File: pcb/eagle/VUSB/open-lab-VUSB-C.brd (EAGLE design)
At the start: 69.5 x 58.4 mm, 70 parts, among them IC1 ATMEGA328P, IC2 MCP73831, IC4 MCP1700-33, IC5 MCP23008, IC6 MAX31855, IC7 ENC28J60, J1 AYZ0202, Q1 BSS123, Q2 BSS123, Q3 BSS123, X1 USBSMD, X2 32.768kHz, X3 25MHz

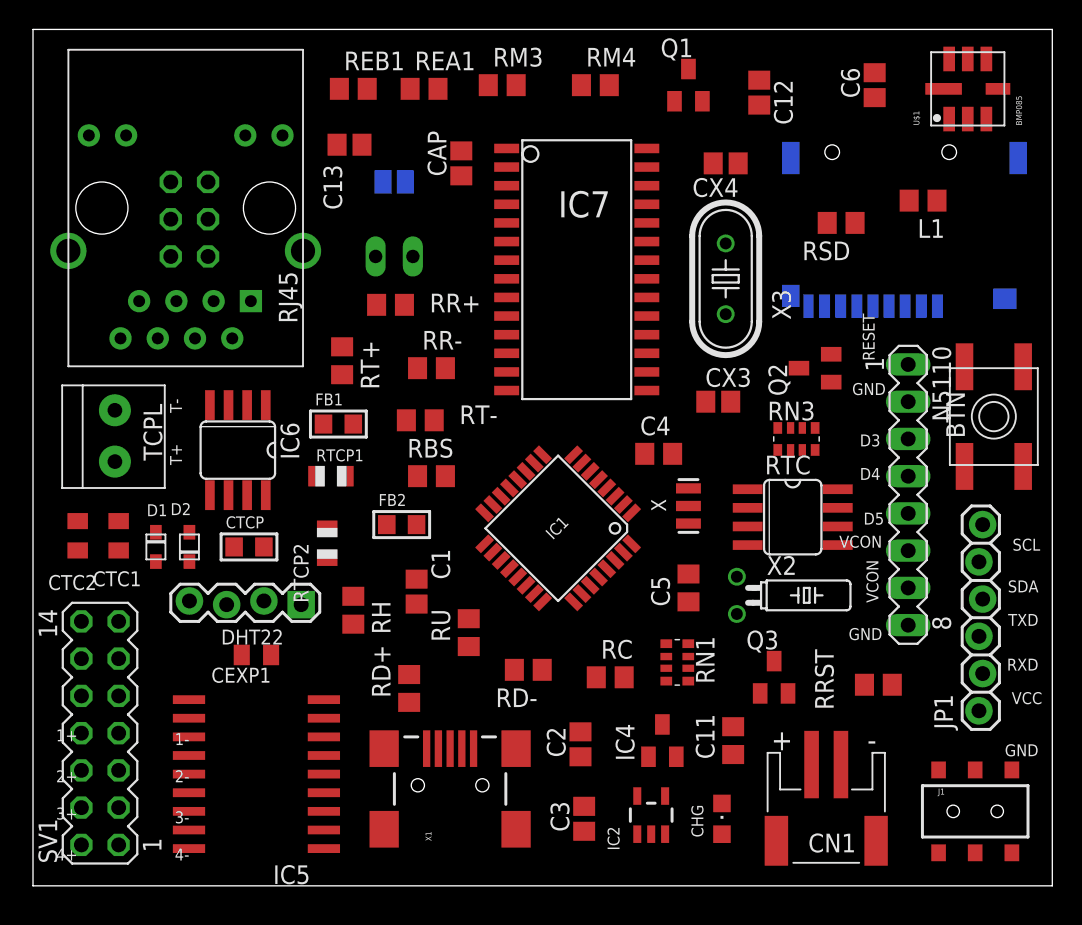
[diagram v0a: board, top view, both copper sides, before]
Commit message: update
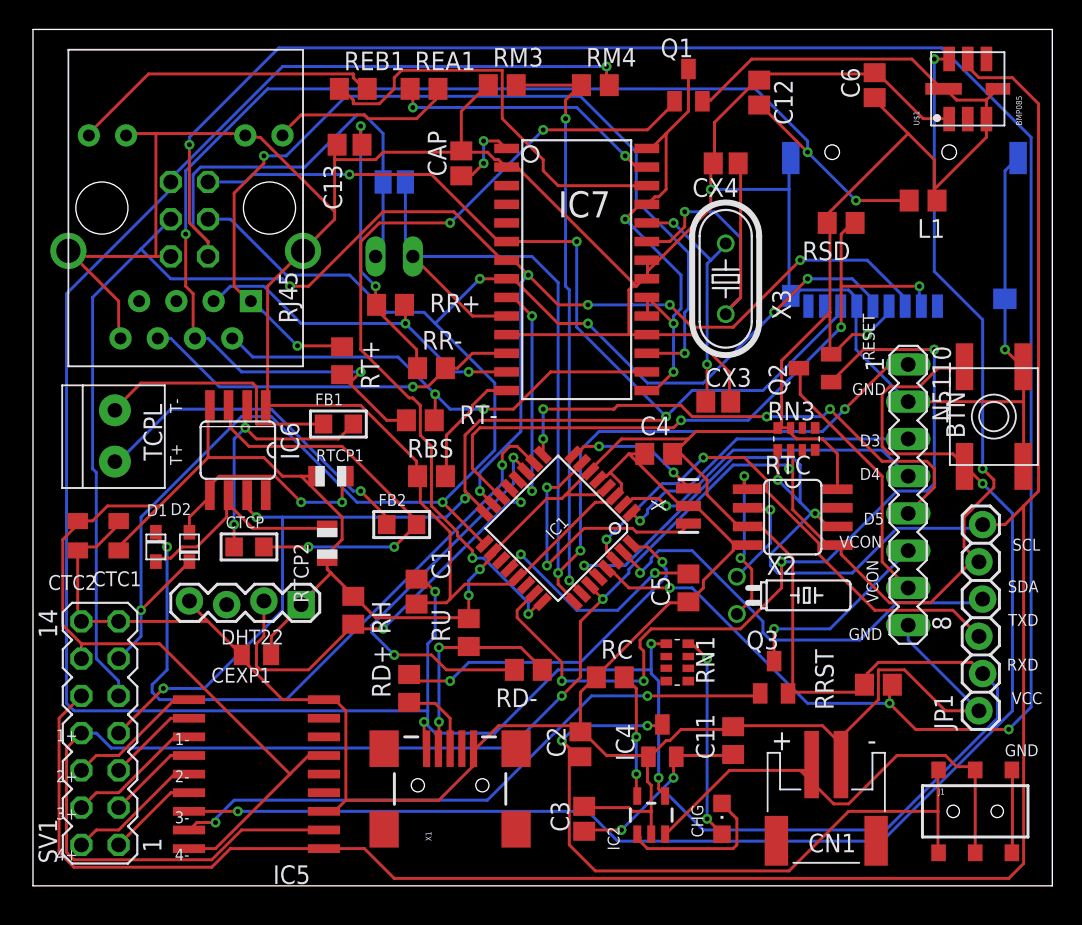
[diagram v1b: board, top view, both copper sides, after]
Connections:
- net GND: now also IC5.4, IC5.5
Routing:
- net GND: track 0.00 -> 391.6 mm, vias 0 -> 2
- net VCC: track 0.00 -> 285.5 mm, vias 0 -> 5
- net SCL: track 0.00 -> 191.3 mm, vias 0 -> 3
- net RESET: track 0.00 -> 175.3 mm, vias 0 -> 4
- net SDA: track 0.00 -> 147.0 mm, vias 0 -> 5
- net VBUS: track 0.00 -> 140.2 mm, vias 0 -> 5
- net SCK: track 0.00 -> 116.7 mm, vias 0 -> 6
- net MISO: track 0.00 -> 114.9 mm, vias 0 -> 6
- net MOSI: track 0.00 -> 114.9 mm, vias 0 -> 6
- net P6: track 0.00 -> 94.9 mm, vias 0 -> 2
- net TCT: track 0.00 -> 91.6 mm, vias 0 -> 4
- net A2: track 0.00 -> 80.0 mm, vias 0 -> 3
- net TD+: track 0.00 -> 65.4 mm, vias 0 -> 3
- net A0: track 0.00 -> 58.8 mm, vias 0 -> 4
- net A1: track 0.00 -> 57.4 mm, vias 0 -> 4
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
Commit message: update
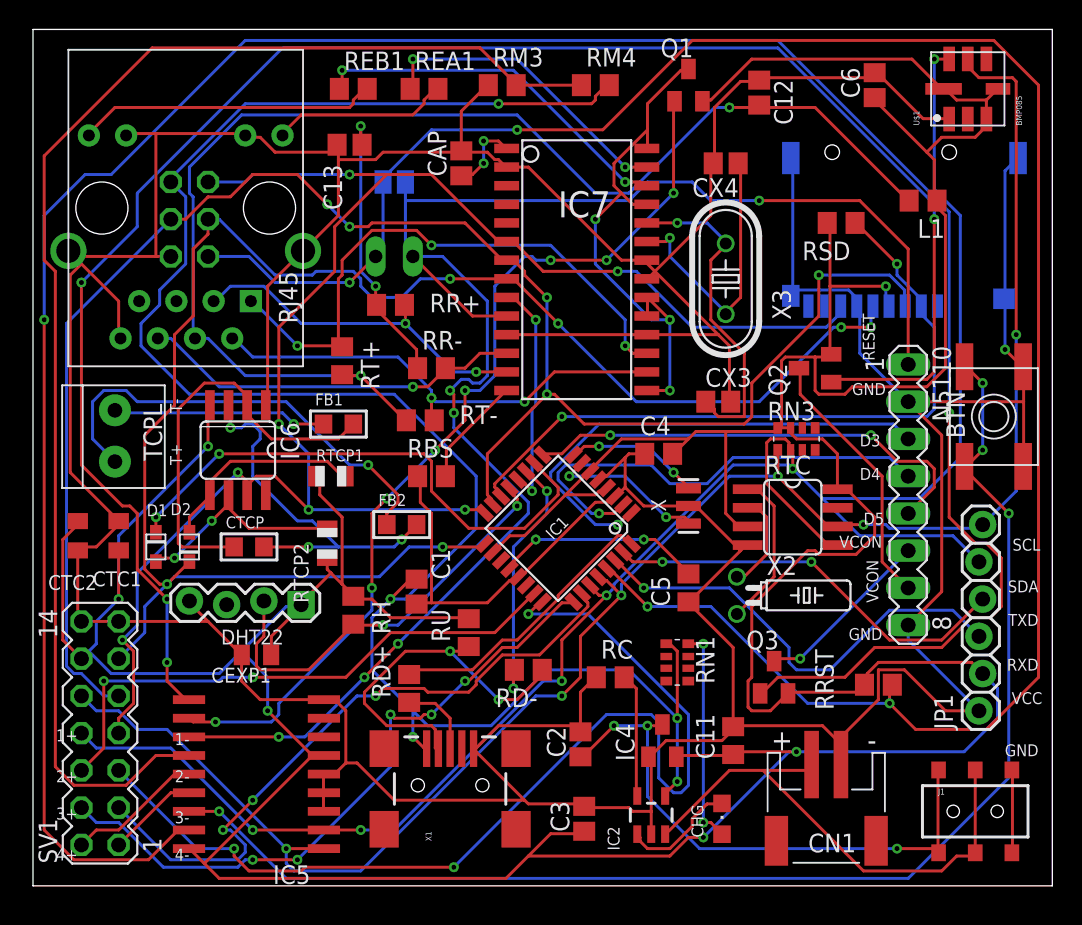
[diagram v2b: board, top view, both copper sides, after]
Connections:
- net A0: now also SV1.6; no longer Q2.1
- net A1: now also SV1.5; no longer Q1.1
- net A2: now also SV1.4; no longer ETHRESET.1, ETHRESETS.2, IC7.10, N5110.1
- net A3: now also SV1.3; no longer RM3.2, RM4.1
- net P0: now also Q2.1; no longer SV1.6
- net P1: now also Q1.1; no longer SV1.5
- net P2: now also ETHRESET.1, ETHRESETS.2, IC7.10, N5110.1; no longer SV1.4
- net P3: now also RM3.2, RM4.1; no longer SV1.3
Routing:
- net P7: track 43.0 -> 172.7 mm
- net P0: track 9.34 -> 121.2 mm, vias 0 -> 4
- net P2: track 9.34 -> 112.6 mm, vias 0 -> 6
- net P3: track 6.27 -> 93.3 mm
- net SCL: track 191.3 -> 123.9 mm, vias 3 -> 6
- net VCC: track 285.5 -> 344.8 mm, vias 5 -> 6
- net P1: track 6.27 -> 63.7 mm, vias 0 -> 8
- net A2: track 80.0 -> 45.1 mm, vias 3 -> 5
- net RESET: track 175.3 -> 145.6 mm
- net GND: track 391.6 -> 419.3 mm, vias 2 -> 1
- net TD+: track 65.4 -> 39.9 mm
- net A0: track 58.8 -> 38.6 mm, vias 4 -> 2
- net SDA: track 147.0 -> 132.8 mm, vias 5 -> 6
- net A1: track 57.4 -> 71.0 mm, vias 4 -> 3
- net D3: track 21.5 -> 33.8 mm
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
